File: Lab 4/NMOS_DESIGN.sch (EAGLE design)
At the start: 22 parts, among them IC3 MAX660CPA, J1 FTDI_DEVICERA_SMT, M1 WIRELESS-NRF24L01, Q1 NTHD3101F, Q2 NTHD3101F, Q3 NTHD3101F, Q4 NTHD3101F, Q5 NTHD3101F, Q6 NTHD3101F, Q7 NTHD3101F, Q8 NTHD3101F, U2 GY-521MPU6050

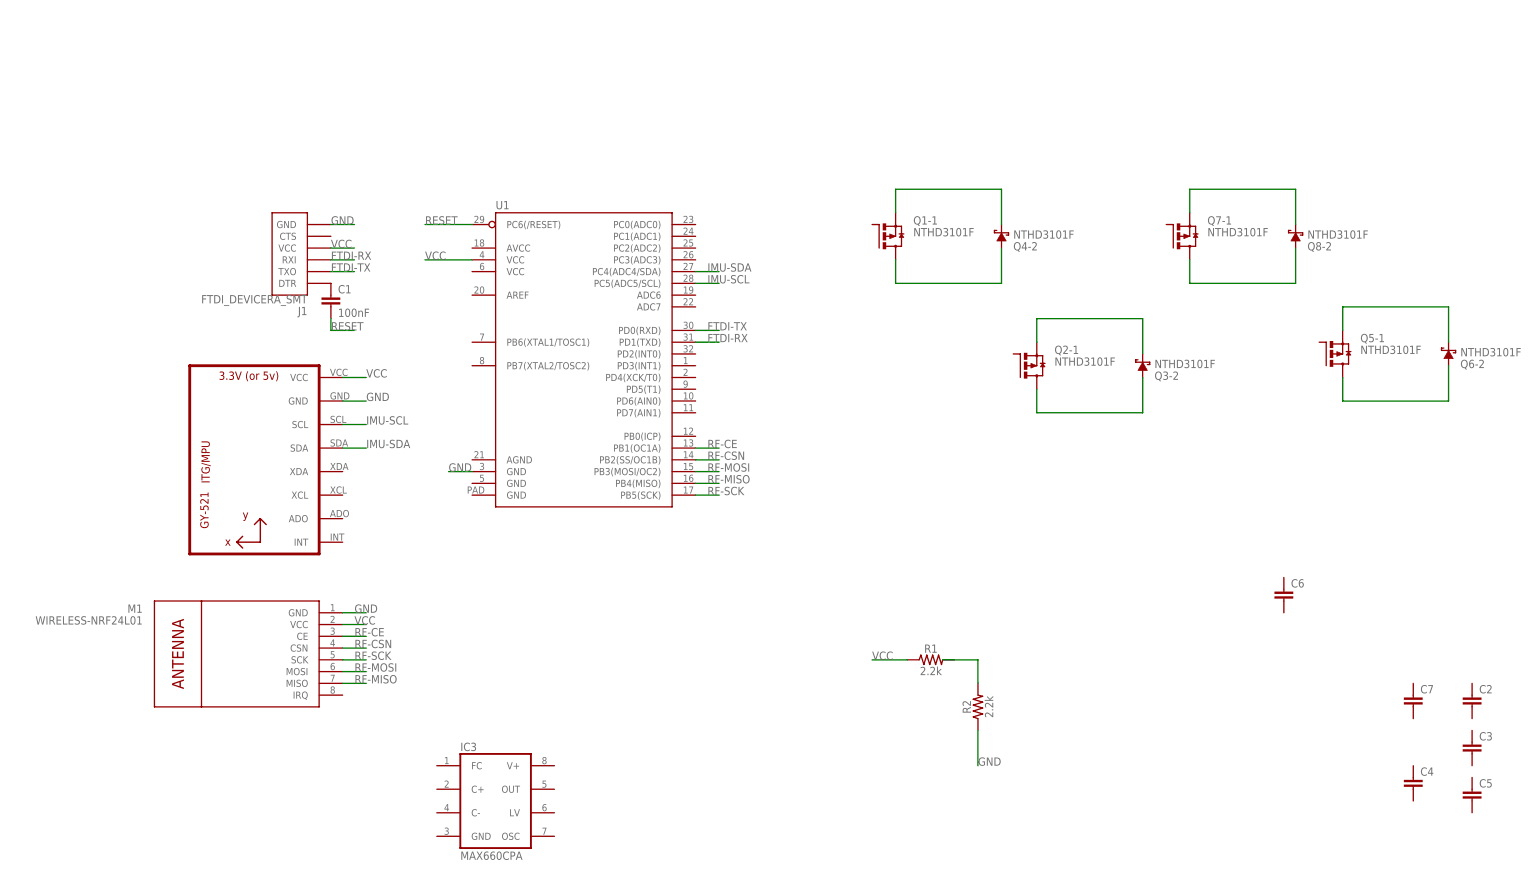
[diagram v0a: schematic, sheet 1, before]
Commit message: Fixed needed on the google sheet
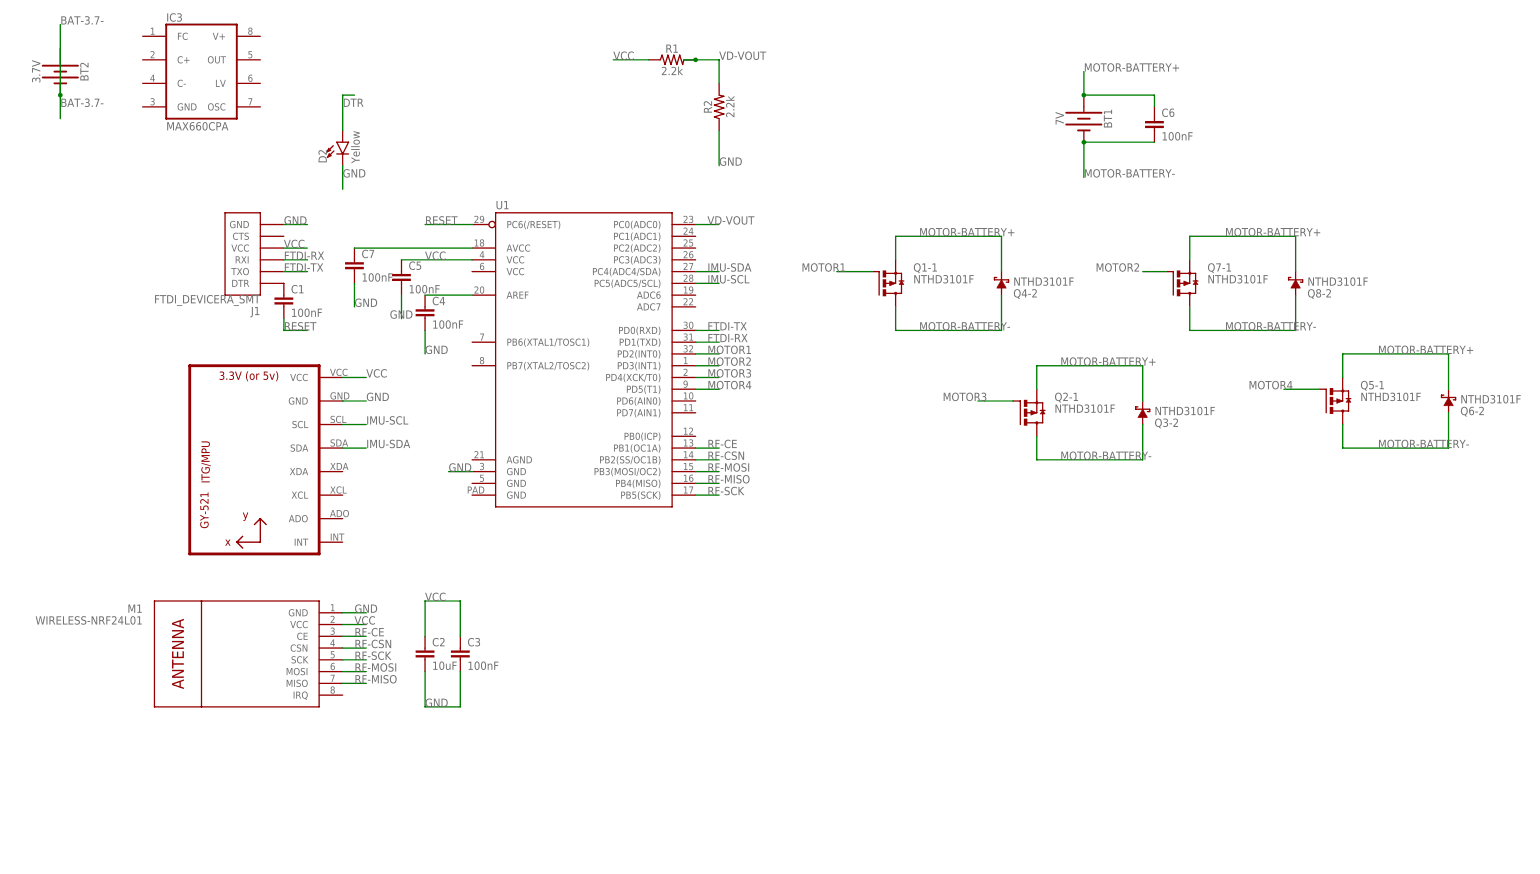
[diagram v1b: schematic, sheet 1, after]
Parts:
- added BT1: 7V, SparkFun-Batteries:BATTERY-9V
- added BT2: 3.7V, SparkFun-Batteries:BATTERY-9V
- added D2: Yellow, SparkFun-LED:LED-YELLOW0603
- C2: value (none) -> 10uF
- C3, C4, C5, C6, C7: value (none) -> 100nF
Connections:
- removed net N$10: Q5-1.D, Q6-2.A
- removed net N$11: Q7-1.S, Q8-2.C
- removed net N$12: Q7-1.D, Q8-2.A
- removed net N$15: R2.2
- removed net N$4: Q1-1.S, Q4-2.C
- removed net N$6: Q1-1.D, Q4-2.A
- removed net N$7: Q2-1.S, Q3-2.C
- removed net N$8: Q2-1.D, Q3-2.A
- removed net N$9: Q5-1.S, Q6-2.C
- new net BAT-3.7-: BT2.+, BT2.-
- new net DTR: D2.A
- new net MOTOR-BATTERY+: BT1.+, C6.1, Q1-1.S, Q2-1.S, Q3-2.C, Q4-2.C, Q5-1.S, Q6-2.C, Q7-1.S, Q8-2.C
- new net MOTOR-BATTERY-: BT1.-, C6.2, Q1-1.D, Q2-1.D, Q3-2.A, Q4-2.A, Q5-1.D, Q6-2.A, Q7-1.D, Q8-2.A
- new net MOTOR1: Q1-1.G, U1.PD2(INT0)
- new net MOTOR2: Q7-1.G, U1.PD3(INT1)
- new net MOTOR3: Q2-1.G, U1.PD4(XCK/T0)
- new net MOTOR4: Q5-1.G, U1.PD5(T1)
- new net N$1: C7.1, U1.AVCC
- new net N$2: C4.1, U1.AREF
- new net VD-VOUT: R1.2, R2.2, U1.PC0(ADC0)
- net GND: now also C2.2, C3.2, C4.2, C5.2, C7.2, D2.C
- net VCC: now also C2.1, C3.1, C5.1
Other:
- moved on the sheet: C1, C2, C3, C4, C5, C6, C7, IC3, J1, Q1-1, Q2-1, Q3-2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
